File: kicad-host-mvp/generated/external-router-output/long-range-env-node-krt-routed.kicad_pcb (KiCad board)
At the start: 2 copper layers, 100 x 68 mm, 6 parts

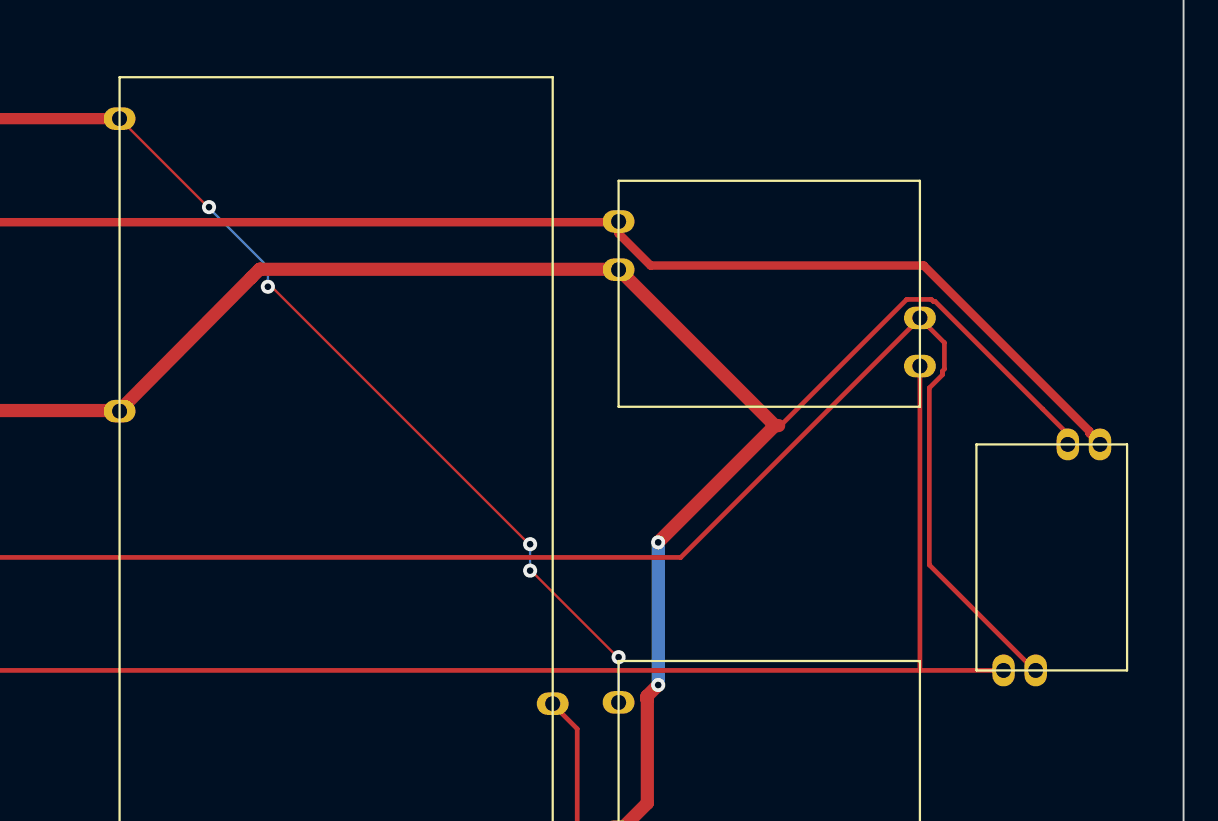
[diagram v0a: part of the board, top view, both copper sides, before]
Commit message: 更新
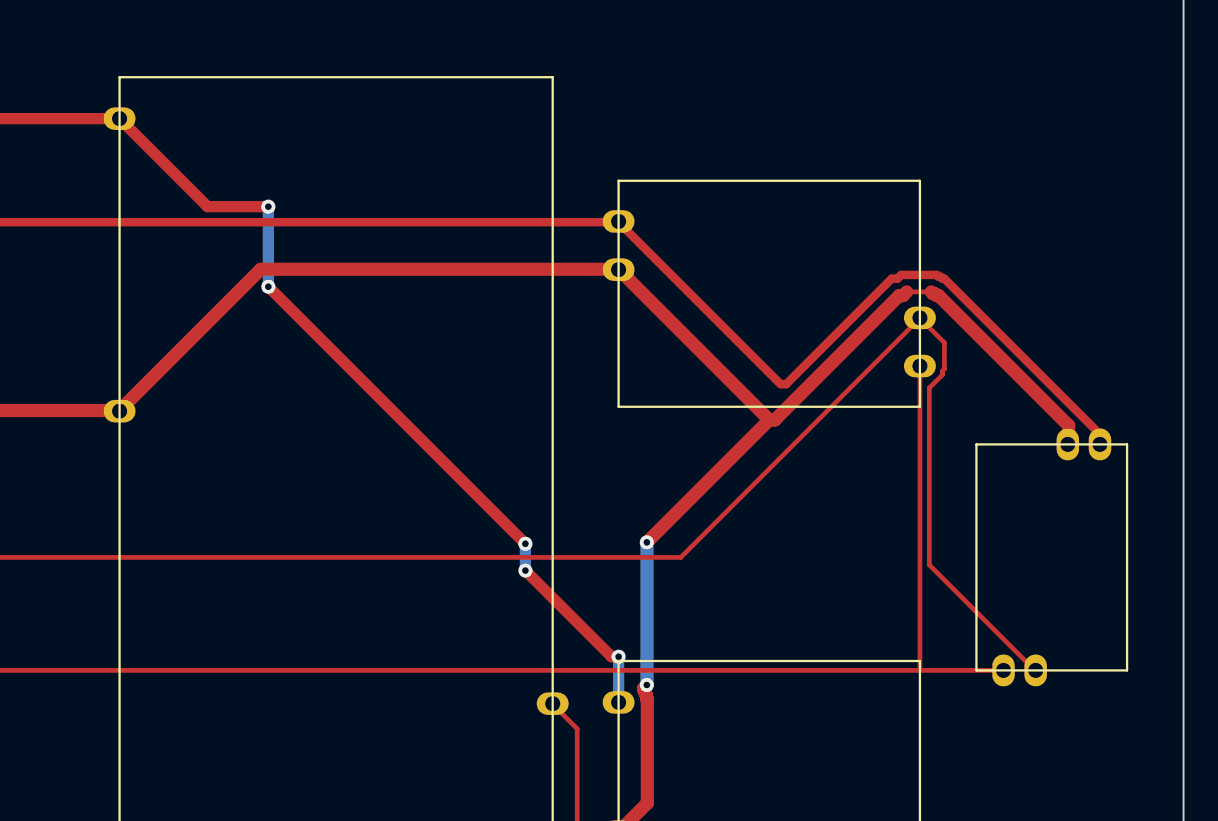
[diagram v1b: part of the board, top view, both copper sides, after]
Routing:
- net 3V3: track 91.4 -> 96.0 mm
- net 5V: track 74.9 -> 77.1 mm
- net GND: track 154.9 -> 155.6 mm

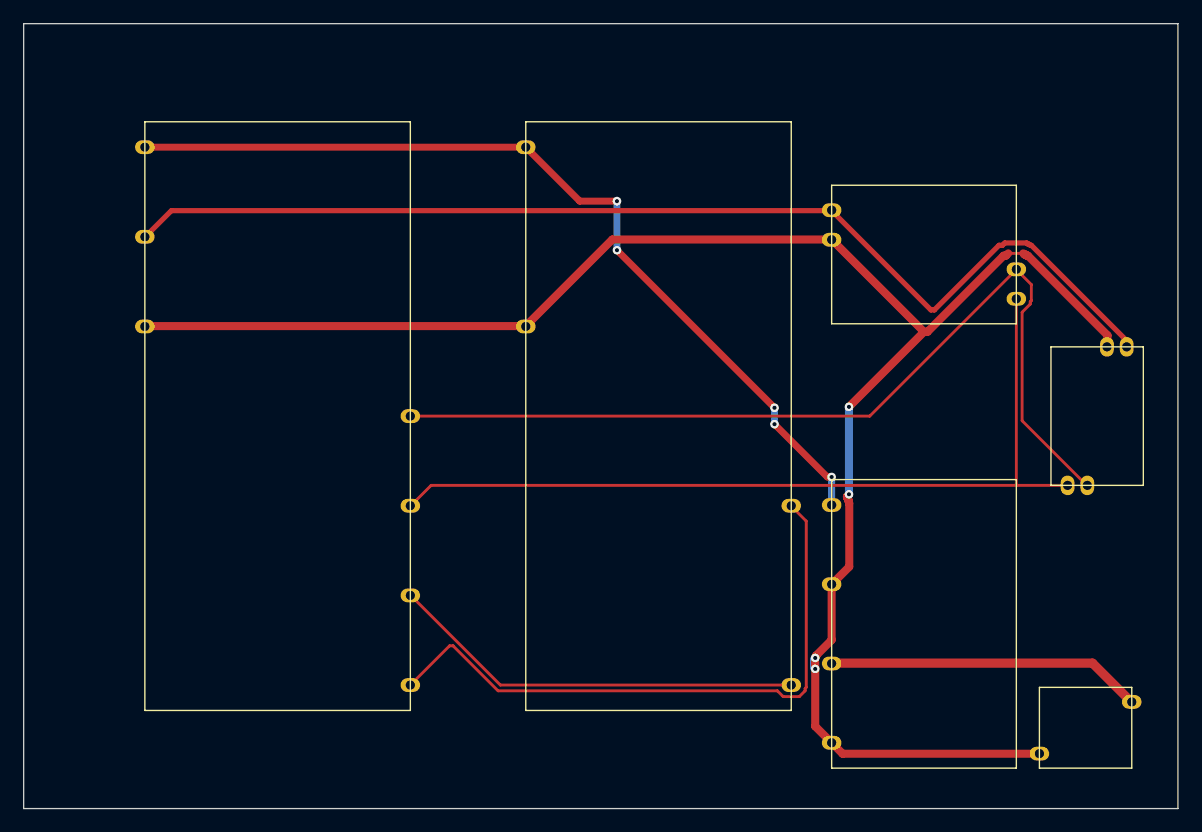
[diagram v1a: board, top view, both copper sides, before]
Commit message: update
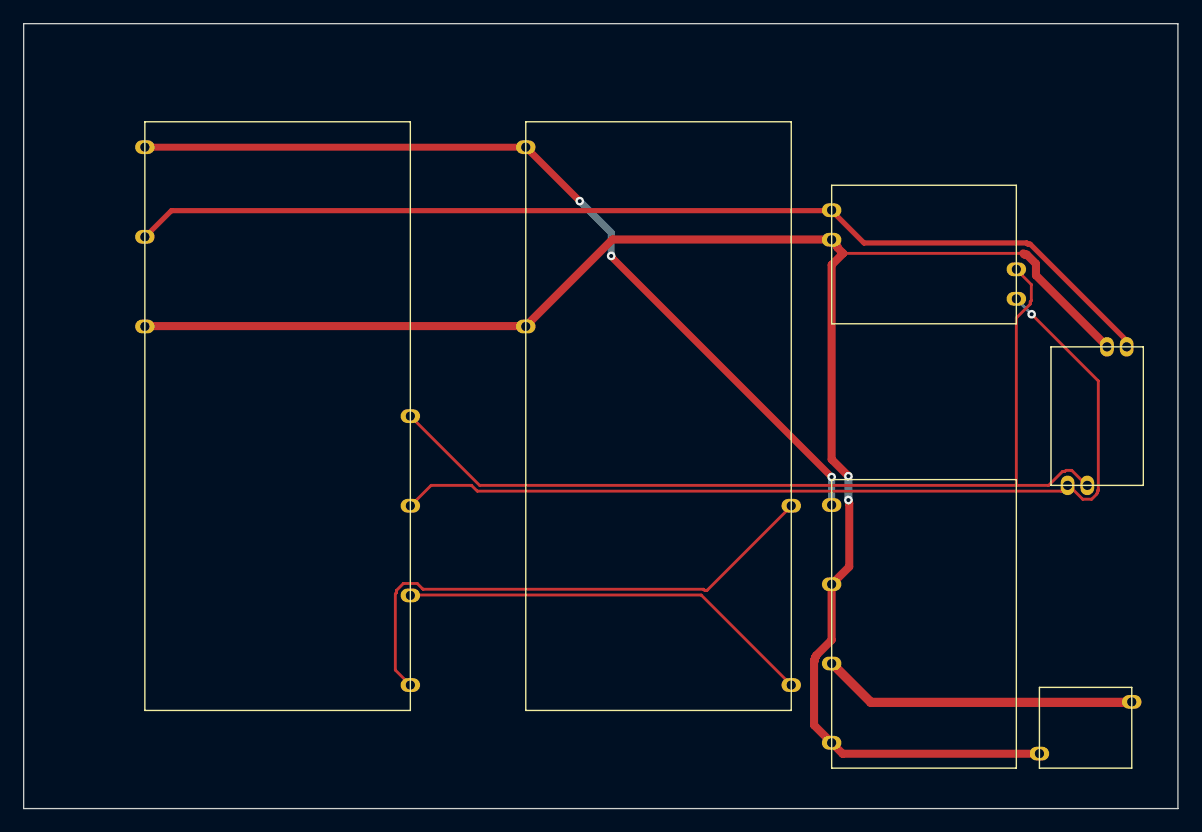
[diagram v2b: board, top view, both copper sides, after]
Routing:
- net LORA_TX: track 54.2 -> 46.5 mm
- net I2C_SCL: track 73.8 -> 81.1 mm, vias 0 -> 1
- net 3V3: track 96.0 -> 91.2 mm
- net I2C_SDA: track 79.6 -> 81.9 mm
- net 5V: track 77.1 -> 74.9 mm, vias 5 -> 3
- net GND: track 155.6 -> 154.7 mm, vias 4 -> 2
